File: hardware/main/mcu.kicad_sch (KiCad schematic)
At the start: 15 parts, among them Q9 SSM3J338R, U1 Holyiot-18010-NRF52840

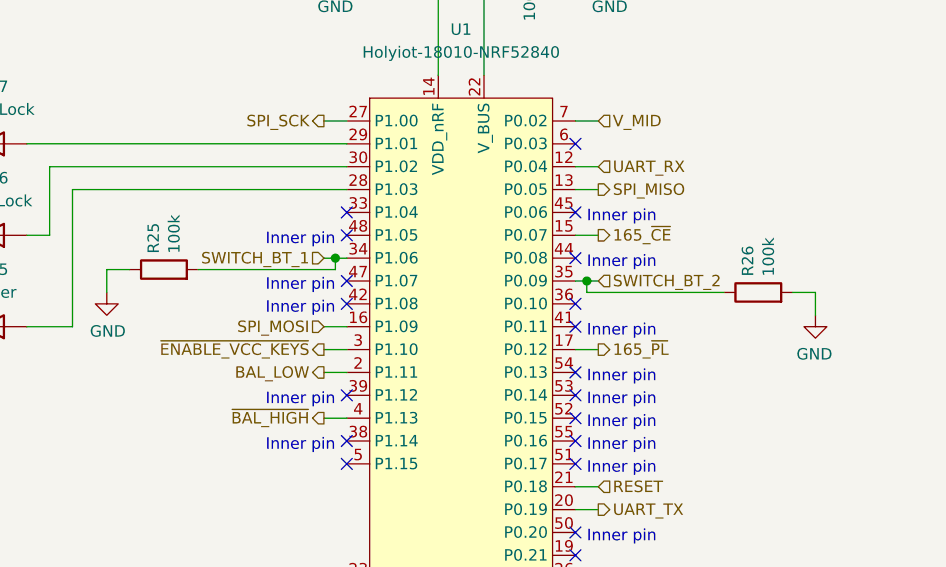
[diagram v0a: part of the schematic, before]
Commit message: Rework the connection to the numpad
Changes:
- The UART lines now have a protection circuit
- The power supply line of the numpad can be switched on and off by the MCU.
- An Id-line is added so that the MCU can detect when the numpad is
  connected.
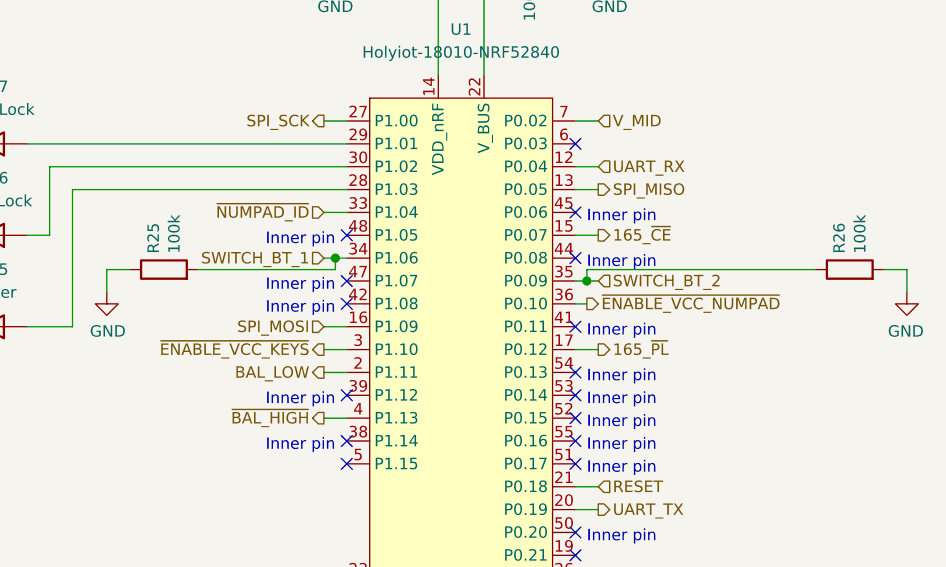
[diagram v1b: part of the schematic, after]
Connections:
- net ~NUMPAD_ID: now reaches U1.33 (P1.04)
- net ~ENABLE_VCC_NUMPAD: now reaches U1.36 (P0.10)
- no-connect marks 26 -> 24
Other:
- moved on the sheet: R26
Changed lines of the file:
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@@
   (junction (at 142.24 29.21) (diameter 1.016) (color 0 0 0 0))
   (junction (at 153.67 67.31) (diameter 1.016) (color 0 0 0 0))
-  (no_connect (at 127 59.69))
   (no_connect (at 127 62.23))
   (no_connect (at 127 67.31))
@@
   (no_connect (at 152.4 59.69))
   (no_connect (at 152.4 64.77))
-  (no_connect (at 152.4 69.85))
   (no_connect (at 152.4 72.39))
   (no_connect (at 152.4 77.47))
@@
     (stroke (width 0) (type solid) (color 0 0 0 0))
   )
+  (wire (pts (xy 124.46 59.69) (xy 127 59.69))
+    (stroke (width 0) (type solid) (color 0 0 0 0))
+  )
   (wire (pts (xy 124.46 64.77) (xy 125.73 64.77))
     (stroke (width 0) (type solid) (color 0 0 0 0))
@@
     (stroke (width 0) (type solid) (color 0 0 0 0))
   )
+  (wire (pts (xy 152.4 69.85) (xy 153.67 69.85))
+    (stroke (width 0) (type solid) (color 0 0 0 0))
+  )
   (wire (pts (xy 152.4 74.93) (xy 154.94 74.93))
     (stroke (width 0) (type solid) (color 0 0 0 0))
@@
     (stroke (width 0) (type solid) (color 0 0 0 0))
   )
+  (wire (pts (xy 153.67 66.04) (xy 153.67 67.31))
+    (stroke (width 0) (type solid) (color 0 0 0 0))
+  )
   (wire (pts (xy 153.67 67.31) (xy 154.94 67.31))
     (stroke (width 0) (type solid) (color 0 0 0 0))
   )
-  (wire (pts (xy 153.67 68.58) (xy 153.67 67.31))
-    (stroke (width 0) (type solid) (color 0 0 0 0))
-  )
   (wire (pts (xy 154.94 29.21) (xy 154.94 31.75))
     (stroke (width 0) (type solid) (color 0 0 0 0))
@@
     (stroke (width 0) (type solid) (color 0 0 0 0))
   )
-  (wire (pts (xy 168.91 68.58) (xy 153.67 68.58))
-    (stroke (width 0) (type solid) (color 0 0 0 0))
-  )
-  (wire (pts (xy 179.07 68.58) (xy 176.53 68.58))
-    (stroke (width 0) (type solid) (color 0 0 0 0))
-  )
-  (wire (pts (xy 179.07 68.58) (xy 179.07 71.12))
+  (wire (pts (xy 179.07 66.04) (xy 153.67 66.04))
+    (stroke (width 0) (type solid) (color 0 0 0 0))
+  )
+  (wire (pts (xy 189.23 66.04) (xy 186.69 66.04))
+    (stroke (width 0) (type solid) (color 0 0 0 0))
+  )
+  (wire (pts (xy 189.23 66.04) (xy 189.23 68.58))
     (stroke (width 0) (type solid) (color 0 0 0 0))
   )
@@
     (effects (font (size 1.27 1.27)) (justify right))
   )
+  (hierarchical_label "~NUMPAD_ID" (shape input) (at 124.46 59.69 180)
+    (effects (font (size 1.27 1.27)) (justify right))
+  )
   (hierarchical_label "SWITCH_BT_1" (shape input) (at 124.46 64.77 180)
     (effects (font (size 1.27 1.27)) (justify right))
@@
   )
   (hierarchical_label "VCC_SW" (shape input) (at 137.16 25.4 90)
+    (effects (font (size 1.27 1.27)) (justify left))
+  )
+  (hierarchical_label "~ENABLE_VCC_NUMPAD" (shape output) (at 153.67 69.85 0)
     (effects (font (size 1.27 1.27)) (justify left))
   )
@@
     )
   )
-  (symbol (lib_id "power:GND") (at 179.07 71.12 0) (mirror y) (unit 1)
-    (in_bom yes) (on_board yes)
-    (property "Reference" "#PWR0149" (id 0) (at 179.07 77.47 0)
-      (effects (font (size 1.27 1.27)) hide)
-    )
-    (property "Value" "GND" (id 1) (at 178.9557 75.4444 0))
-    (property "Footprint" "" (id 2) (at 179.07 71.12 0)
-      (effects (font (size 1.27 1.27)) hide)
-    )
-    (property "Datasheet" "" (id 3) (at 179.07 71.12 0)
+  (symbol (lib_id "power:GND") (at 189.23 68.58 0) (mirror y) (unit 1)
+    (in_bom yes) (on_board yes)
+    (property "Reference" "#PWR0149" (id 0) (at 189.23 74.93 0)
+      (effects (font (size 1.27 1.27)) hide)
+    )
+    (property "Value" "GND" (id 1) (at 189.1157 72.9044 0))
+    (property "Footprint" "" (id 2) (at 189.23 68.58 0)
+      (effects (font (size 1.27 1.27)) hide)
+    )
+    (property "Datasheet" "" (id 3) (at 189.23 68.58 0)
       (effects (font (size 1.27 1.27)) hide)
     )
@@
     )
   )
-  (symbol (lib_id "Device:R") (at 172.72 68.58 90) (unit 1)
-    (in_bom yes) (on_board yes)
-    (property "Reference" "R26" (id 0) (at 171.5706 66.8019 0)
-      (effects (font (size 1.27 1.27)) (justify left))
-    )
-    (property "Value" "100k" (id 1) (at 173.8693 66.8019 0)
-      (effects (font (size 1.27 1.27)) (justify left))
-    )
-    (property "Footprint" "Resistor_SMD:R_0603_1608Metric_Pad0.98x0.95mm_HandSolder" (id 2) (at 172.72 70.358 90)
-      (effects (font (size 1.27 1.27)) hide)
-    )
-    (property "Datasheet" "~" (id 3) (at 172.72 68.58 0)
-      (effects (font (size 1.27 1.27)) hide)
-    )
+  (symbol (lib_id "Device:R") (at 182.88 66.04 90) (unit 1)
+    (in_bom yes) (on_board yes)
+    (property "Reference" "R26" (id 0) (at 181.7306 64.2619 0)
+      (effects (font (size 1.27 1.27)) (justify left))
+    )
+    (property "Value" "100k" (id 1) (at 184.0293 64.2619 0)
+      (effects (font (size 1.27 1.27)) (justify left))
+    )
+    (property "Footprint" "Resistor_SMD:R_0603_1608Metric_Pad0.98x0.95mm_HandSolder" (id 2) (at 182.88 67.818 90)
+      (effects (font (size 1.27 1.27)) hide)
+    )
+    (property "Datasheet" "~" (id 3) (at 182.88 66.04 0)
+      (effects (font (size 1.27 1.27)) hide)
+    )

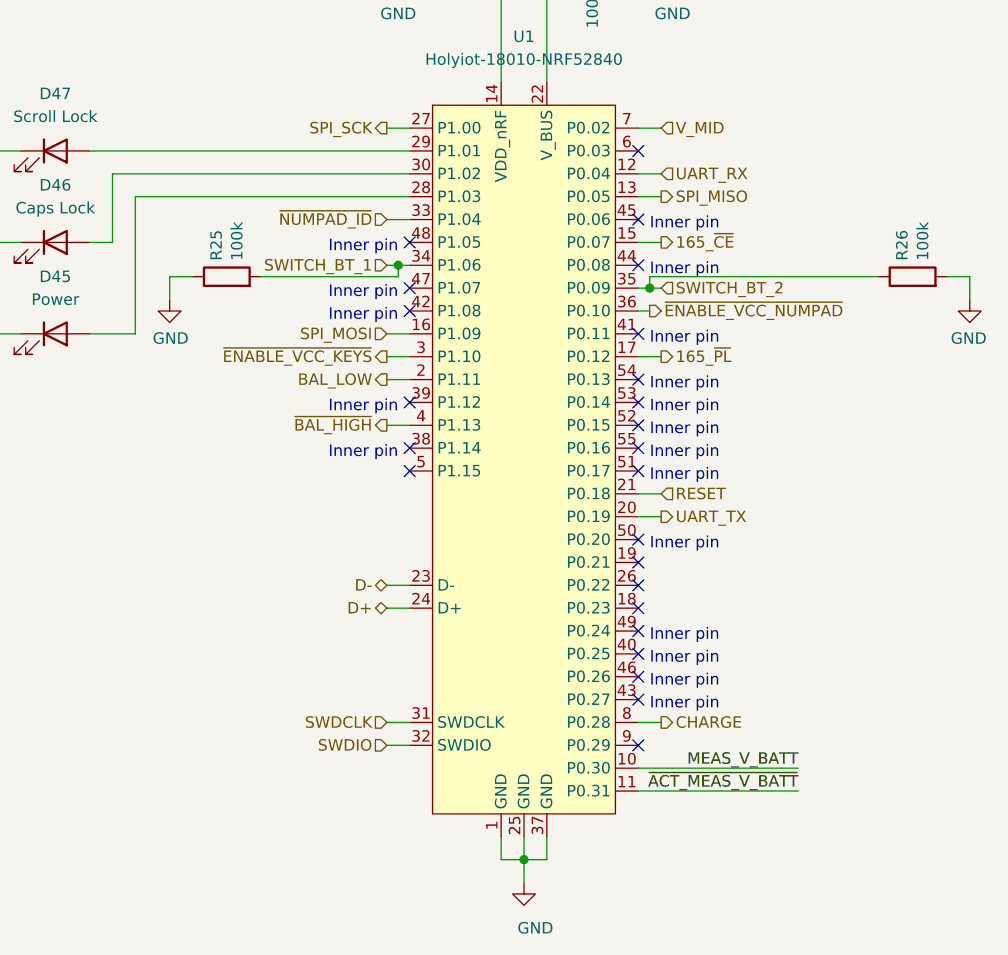
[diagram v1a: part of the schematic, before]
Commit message: WIP: Design of PCB
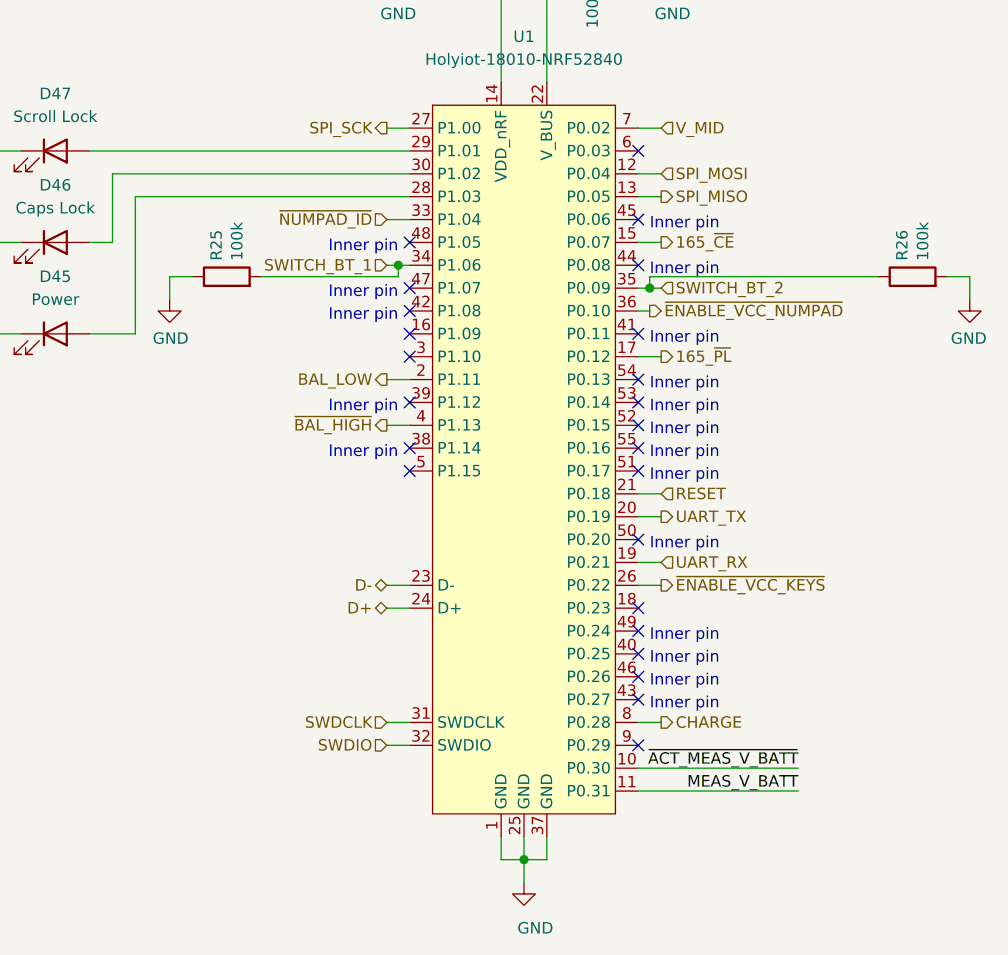
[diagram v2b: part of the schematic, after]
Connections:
- net MEAS_V_BATT: now also U1.11 (P0.31); no longer U1.10 (P0.30)
- net SPI_MOSI: now also U1.12 (P0.04); no longer U1.16 (P1.09)
- net UART_RX: now also U1.19 (P0.21); no longer U1.12 (P0.04)
- net ~ACT_MEAS_V_BATT: now also U1.10 (P0.30); no longer U1.11 (P0.31)
- net ~ENABLE_VCC_KEYS: now also U1.26 (P0.22); no longer U1.3 (P1.10)
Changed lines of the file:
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@@
   (no_connect (at 127 67.31))
   (no_connect (at 127 69.85))
+  (no_connect (at 127 72.39))
+  (no_connect (at 127 74.93))
   (no_connect (at 127 80.01))
   (no_connect (at 127 85.09))
@@
   (no_connect (at 152.4 87.63))
   (no_connect (at 152.4 95.25))
-  (no_connect (at 152.4 97.79))
-  (no_connect (at 152.4 100.33))
   (no_connect (at 152.4 102.87))
   (no_connect (at 152.4 105.41))
@@
     (stroke (width 0) (type solid) (color 0 0 0 0))
   )
-  (wire (pts (xy 124.46 72.39) (xy 127 72.39))
-    (stroke (width 0) (type solid) (color 0 0 0 0))
-  )
-  (wire (pts (xy 124.46 74.93) (xy 127 74.93))
-    (stroke (width 0) (type solid) (color 0 0 0 0))
-  )
   (wire (pts (xy 124.46 77.47) (xy 127 77.47))
     (stroke (width 0) (type solid) (color 0 0 0 0))
@@
     (stroke (width 0) (type solid) (color 0 0 0 0))
   )
+  (wire (pts (xy 152.4 100.33) (xy 154.94 100.33))
+    (stroke (width 0) (type solid) (color 0 0 0 0))
+  )
   (wire (pts (xy 152.4 115.57) (xy 154.94 115.57))
     (stroke (width 0) (type solid) (color 0 0 0 0))
@@
   )
   (wire (pts (xy 154.94 57.15) (xy 152.4 57.15))
+    (stroke (width 0) (type solid) (color 0 0 0 0))
+  )
+  (wire (pts (xy 154.94 97.79) (xy 152.4 97.79))
     (stroke (width 0) (type solid) (color 0 0 0 0))
   )
@@
     (effects (font (size 1.27 1.27)) (justify right bottom))
   )
-  (label "MEAS_V_BATT" (at 170.18 120.65 180)
-    (effects (font (size 1.27 1.27)) (justify right bottom))
-  )
-  (label "~ACT_MEAS_V_BATT" (at 170.18 123.19 180)
+  (label "~ACT_MEAS_V_BATT" (at 170.18 120.65 180)
+    (effects (font (size 1.27 1.27)) (justify right bottom))
+  )
+  (label "MEAS_V_BATT" (at 170.18 123.19 180)
     (effects (font (size 1.27 1.27)) (justify right bottom))
   )
@@
     (effects (font (size 1.27 1.27)) (justify right))
   )
-  (hierarchical_label "SPI_MOSI" (shape input) (at 124.46 72.39 180)
-    (effects (font (size 1.27 1.27)) (justify right))
-  )
-  (hierarchical_label "~ENABLE_VCC_KEYS" (shape output) (at 124.46 74.93 180)
-    (effects (font (size 1.27 1.27)) (justify right))
-  )
   (hierarchical_label "BAL_LOW" (shape output) (at 124.46 77.47 180)
     (effects (font (size 1.27 1.27)) (justify right))
@@
     (effects (font (size 1.27 1.27)) (justify left))
   )
-  (hierarchical_label "UART_RX" (shape input) (at 154.94 54.61 0)
+  (hierarchical_label "SPI_MOSI" (shape input) (at 154.94 54.61 0)
     (effects (font (size 1.27 1.27)) (justify left))
   )
@@
     (effects (font (size 1.27 1.27)) (justify left))
   )
+  (hierarchical_label "UART_RX" (shape input) (at 154.94 97.79 0)
+    (effects (font (size 1.27 1.27)) (justify left))
+  )
+  (hierarchical_label "~ENABLE_VCC_KEYS" (shape output) (at 154.94 100.33 0)
+    (effects (font (size 1.27 1.27)) (justify left))
+  )

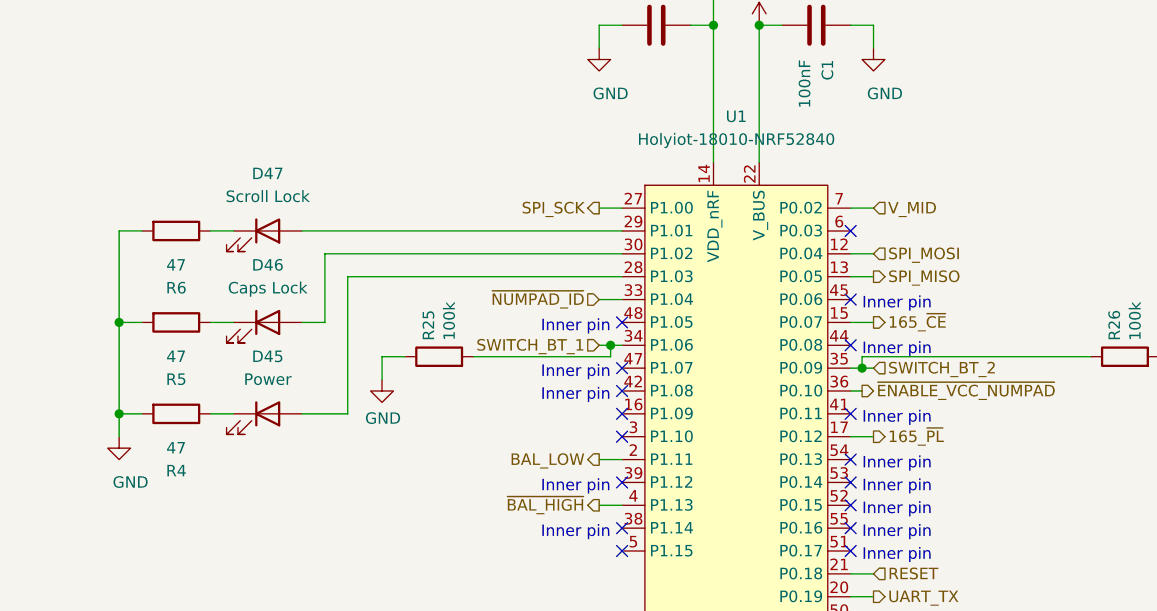
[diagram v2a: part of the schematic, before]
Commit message: WIP: Design of PCB
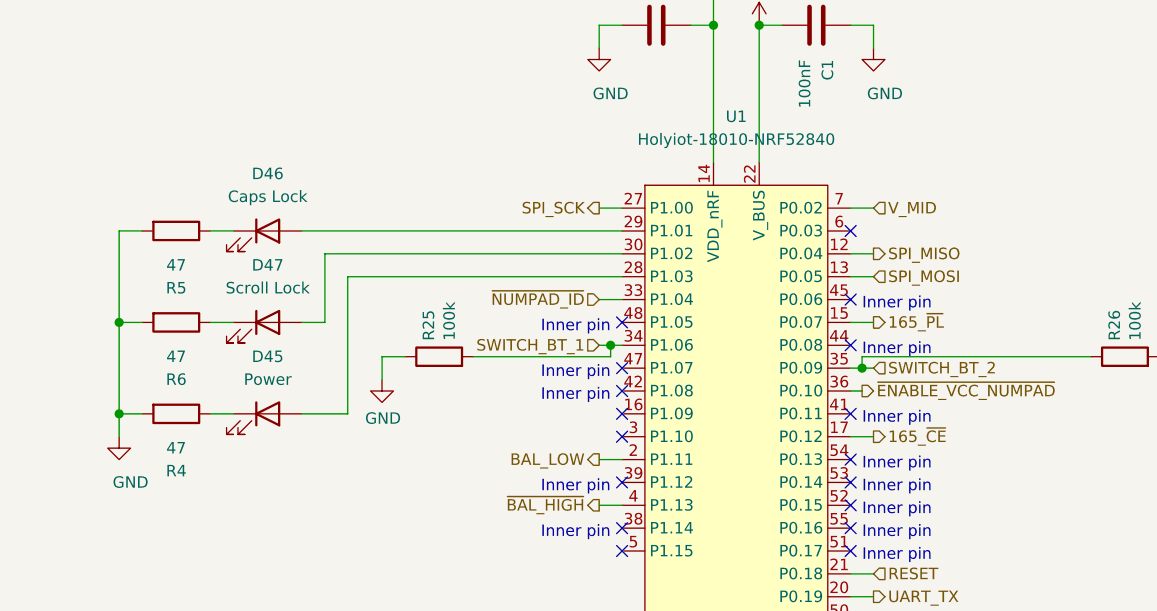
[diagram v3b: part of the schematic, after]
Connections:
- net 165_~CE: now also U1.17 (P0.12); no longer U1.15 (P0.07)
- net 165_~PL: now also U1.15 (P0.07); no longer U1.17 (P0.12)
- net SPI_MISO: now also U1.12 (P0.04); no longer U1.13 (P0.05)
- net SPI_MOSI: now also U1.13 (P0.05); no longer U1.12 (P0.04)
- net at D47.2 (A): now also U1.30 (P1.02); no longer U1.29 (P1.01)
- net at D46.2 (A): now also U1.29 (P1.01); no longer U1.30 (P1.02)
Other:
- moved on the sheet: D46, D47, R5, R6
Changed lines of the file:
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@@
     (effects (font (size 1.27 1.27)) (justify left))
   )
-  (hierarchical_label "SPI_MOSI" (shape input) (at 154.94 54.61 0)
-    (effects (font (size 1.27 1.27)) (justify left))
-  )
-  (hierarchical_label "SPI_MISO" (shape output) (at 154.94 57.15 0)
-    (effects (font (size 1.27 1.27)) (justify left))
-  )
-  (hierarchical_label "165_~CE" (shape output) (at 154.94 62.23 0)
+  (hierarchical_label "SPI_MISO" (shape output) (at 154.94 54.61 0)
+    (effects (font (size 1.27 1.27)) (justify left))
+  )
+  (hierarchical_label "SPI_MOSI" (shape input) (at 154.94 57.15 0)
+    (effects (font (size 1.27 1.27)) (justify left))
+  )
+  (hierarchical_label "165_~PL" (shape output) (at 154.94 62.23 0)
     (effects (font (size 1.27 1.27)) (justify left))
   )
@@
     (effects (font (size 1.27 1.27)) (justify left))
   )
-  (hierarchical_label "165_~PL" (shape output) (at 154.94 74.93 0)
+  (hierarchical_label "165_~CE" (shape output) (at 154.94 74.93 0)
     (effects (font (size 1.27 1.27)) (justify left))
   )
@@
   (symbol (lib_id "Device:R") (at 77.47 52.07 270) (unit 1)
     (in_bom yes) (on_board yes)
-    (property "Reference" "R6" (id 0) (at 77.47 58.42 90))
+    (property "Reference" "R5" (id 0) (at 77.47 58.42 90))
     (property "Value" "47" (id 1) (at 77.47 55.88 90))
     (property "Footprint" "Resistor_SMD:R_0603_1608Metric_Pad0.98x0.95mm_HandSolder" (id 2) (at 77.47 50.292 90)
@@
   (symbol (lib_id "Device:R") (at 77.47 62.23 270) (unit 1)
     (in_bom yes) (on_board yes)
-    (property "Reference" "R5" (id 0) (at 77.47 68.58 90))
+    (property "Reference" "R6" (id 0) (at 77.47 68.58 90))
     (property "Value" "47" (id 1) (at 77.47 66.04 90))
     (property "Footprint" "Resistor_SMD:R_0603_1608Metric_Pad0.98x0.95mm_HandSolder" (id 2) (at 77.47 60.452 90)
@@
   (symbol (lib_id "Device:LED") (at 87.63 52.07 0) (unit 1)
     (in_bom yes) (on_board yes)
-    (property "Reference" "D47" (id 0) (at 87.63 45.72 0))
-    (property "Value" "Scroll Lock" (id 1) (at 87.63 48.26 0))
+    (property "Reference" "D46" (id 0) (at 87.63 45.72 0))
+    (property "Value" "Caps Lock" (id 1) (at 87.63 48.26 0))
     (property "Footprint" "Diode_SMD:D_0603_1608Metric_Pad1.05x0.95mm_HandSolder" (id 2) (at 87.63 52.07 0)
       (effects (font (size 1.27 1.27)) hide)
@@
   (symbol (lib_id "Device:LED") (at 87.63 62.23 0) (unit 1)
     (in_bom yes) (on_board yes)
-    (property "Reference" "D46" (id 0) (at 87.63 55.88 0))
-    (property "Value" "Caps Lock" (id 1) (at 87.63 58.42 0))
+    (property "Reference" "D47" (id 0) (at 87.63 55.88 0))
+    (property "Value" "Scroll Lock" (id 1) (at 87.63 58.42 0))
     (property "Footprint" "Diode_SMD:D_0603_1608Metric_Pad1.05x0.95mm_HandSolder" (id 2) (at 87.63 62.23 0)
       (effects (font (size 1.27 1.27)) hide)
